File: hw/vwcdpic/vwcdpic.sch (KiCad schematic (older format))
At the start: 12 parts, among them U1 PIC12F629, U2 LM78L05ACZ, U3 MC78L05ACH

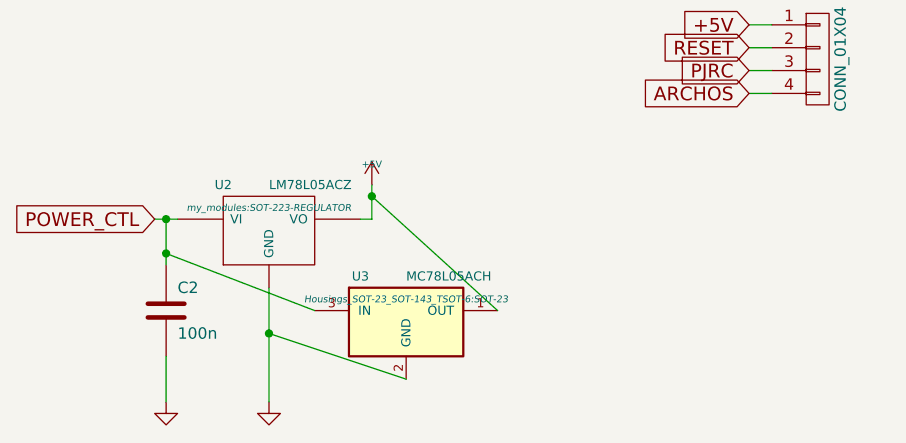
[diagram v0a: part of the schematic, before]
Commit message: update, new schematics file
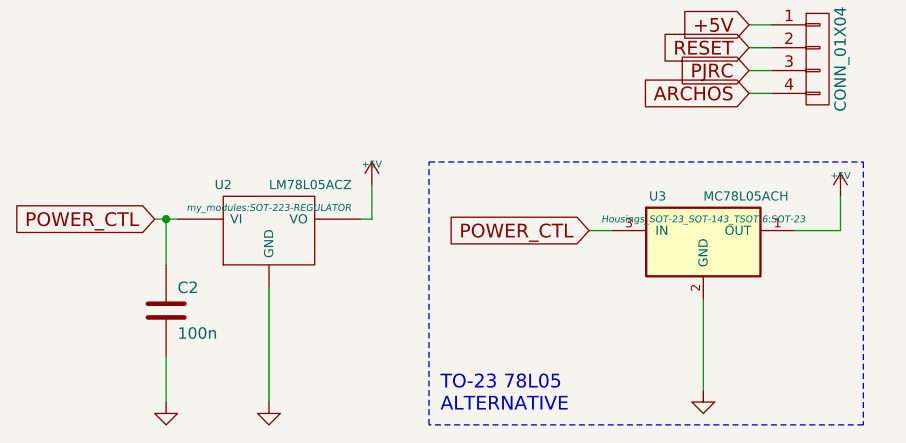
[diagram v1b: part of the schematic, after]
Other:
- note added: "TO-23 78L05\nALTERNATIVE"
- moved on the sheet: U3
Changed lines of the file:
@@
 LIBS:phonejack
 LIBS:device_sot
-LIBS:vwcdpic-rescue
 LIBS:vwcdpic-cache
 EELAYER 25 0
@@
 L MC78L05ACH U3
 U 1 1 561664C4
-P 6100 5600
-F 0 "U3" H 5900 5800 40  0000 C CNN
-F 1 "MC78L05ACH" H 6100 5800 40  0000 L CNN
-F 2 "Housings_SOT-23_SOT-143_TSOT-6:SOT-23" H 6100 5700 30  0000 C CIN
-F 3 "" H 6100 5600 60  0000 C CNN
-	1    6100 5600
+P 7400 5250
+F 0 "U3" H 7200 5450 40  0000 C CNN
+F 1 "MC78L05ACH" H 7400 5450 40  0000 L CNN
+F 2 "Housings_SOT-23_SOT-143_TSOT-6:SOT-23" H 7400 5350 30  0000 C CIN
+F 3 "" H 7400 5250 60  0000 C CNN
+	1    7400 5250
 	1    0    0    -1
 $EndComp
@@
 Wire Wire Line
 	7600 4300 7700 4300
-Wire Wire Line
-	5700 5550 5050 5300
-Connection ~ 5050 5300
-Wire Wire Line
-	6100 5850 5500 5650
-Connection ~ 5500 5650
-Wire Wire Line
-	6500 5550 5950 5050
-Connection ~ 5950 5050
+$Comp
+L +5V #PWR?
+U 1 1 5617A229
+P 8000 5050
+F 0 "#PWR?" H 8000 5140 20  0001 C CNN
+F 1 "+5V" H 8000 5140 30  0000 C CNN
+F 2 "" H 8000 5050 60  0001 C CNN
+F 3 "" H 8000 5050 60  0001 C CNN
+	1    8000 5050
+	1    0    0    -1
+$EndComp
+Text GLabel 6900 5200 0    60   Input ~ 0
+POWER_CTL
+$Comp
+L GND #PWR?
+U 1 1 5617A2CE
+P 7400 5900
+F 0 "#PWR?" H 7400 5900 30  0001 C CNN
+F 1 "GND" H 7400 5830 30  0001 C CNN
+F 2 "" H 7400 5900 60  0001 C CNN
+F 3 "" H 7400 5900 60  0001 C CNN
+	1    7400 5900
+	1    0    0    -1
+$EndComp
+Wire Wire Line
+	8000 5050 8000 5200
+Wire Wire Line
+	8000 5200 7800 5200
+Wire Wire Line
+	7000 5200 6900 5200
+Wire Wire Line
+	7400 5900 7400 5500
+Wire Notes Line
+	6200 4900 8100 4900
+Wire Notes Line
+	8100 4900 8100 6050
+Wire Notes Line
+	8100 6050 6200 6050
+Wire Notes Line
+	6200 6050 6200 4900
+Text Notes 6250 6000 0    60   ~ 0
+TO-23 78L05\nALTERNATIVE
 $EndSCHEMATC
